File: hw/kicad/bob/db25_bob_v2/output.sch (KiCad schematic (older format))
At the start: 6 parts, among them P5 CONN_01X08, P6 CONN_01X08, P7 CONN_01X08, P8 CONN_01X08, U18 NCV7608, U19 NCV7608

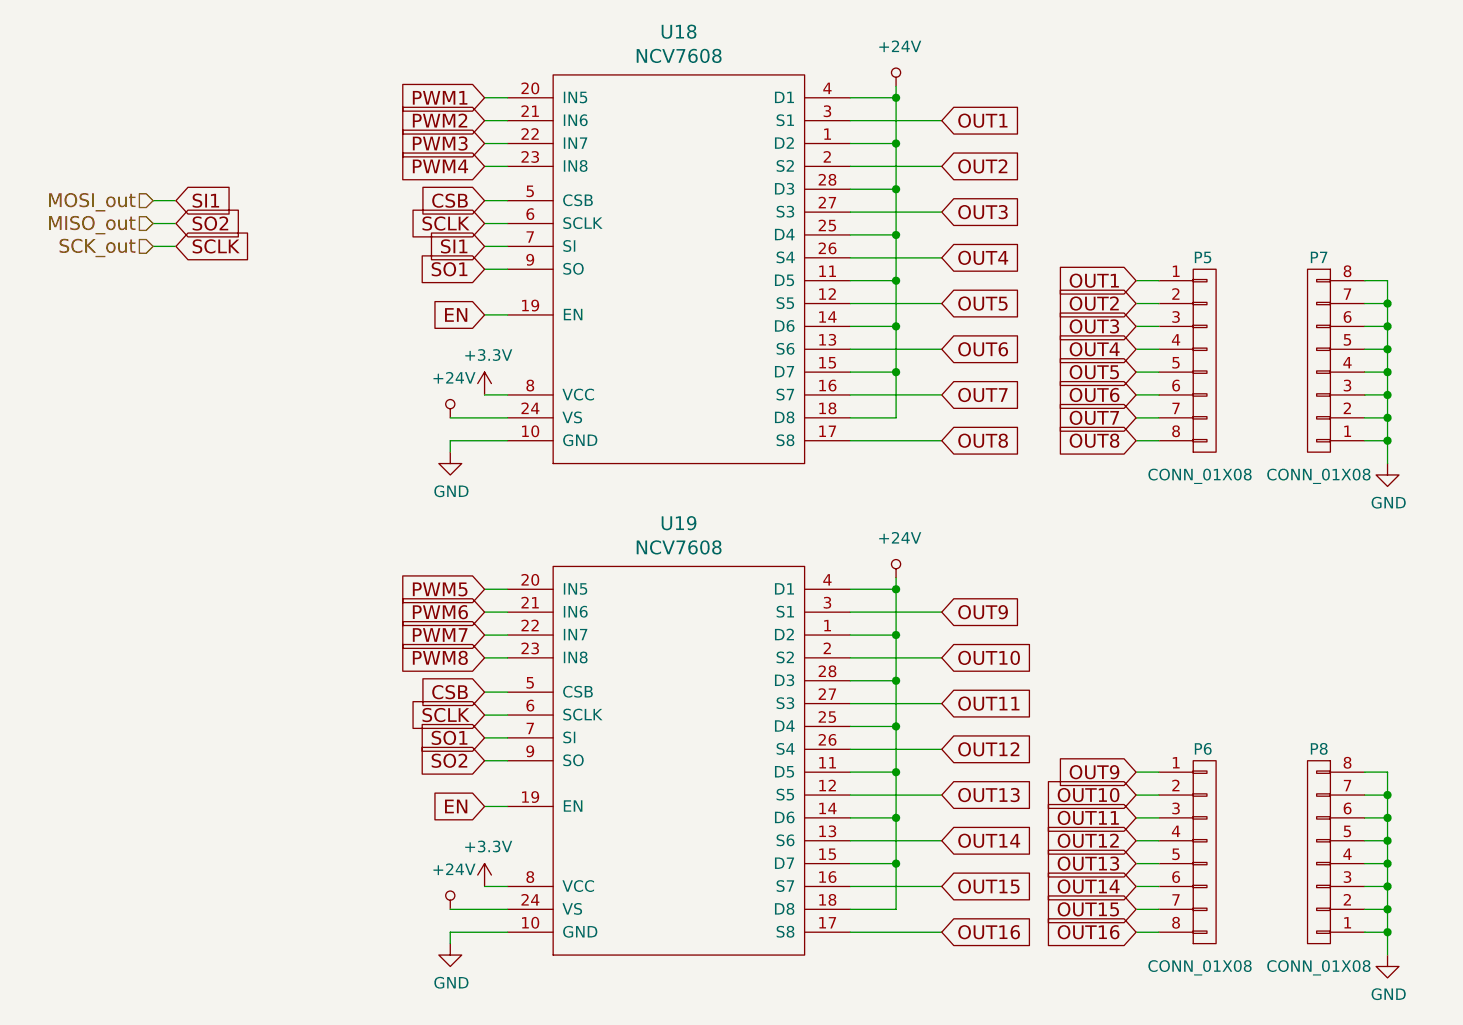
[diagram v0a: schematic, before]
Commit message: More stuff.
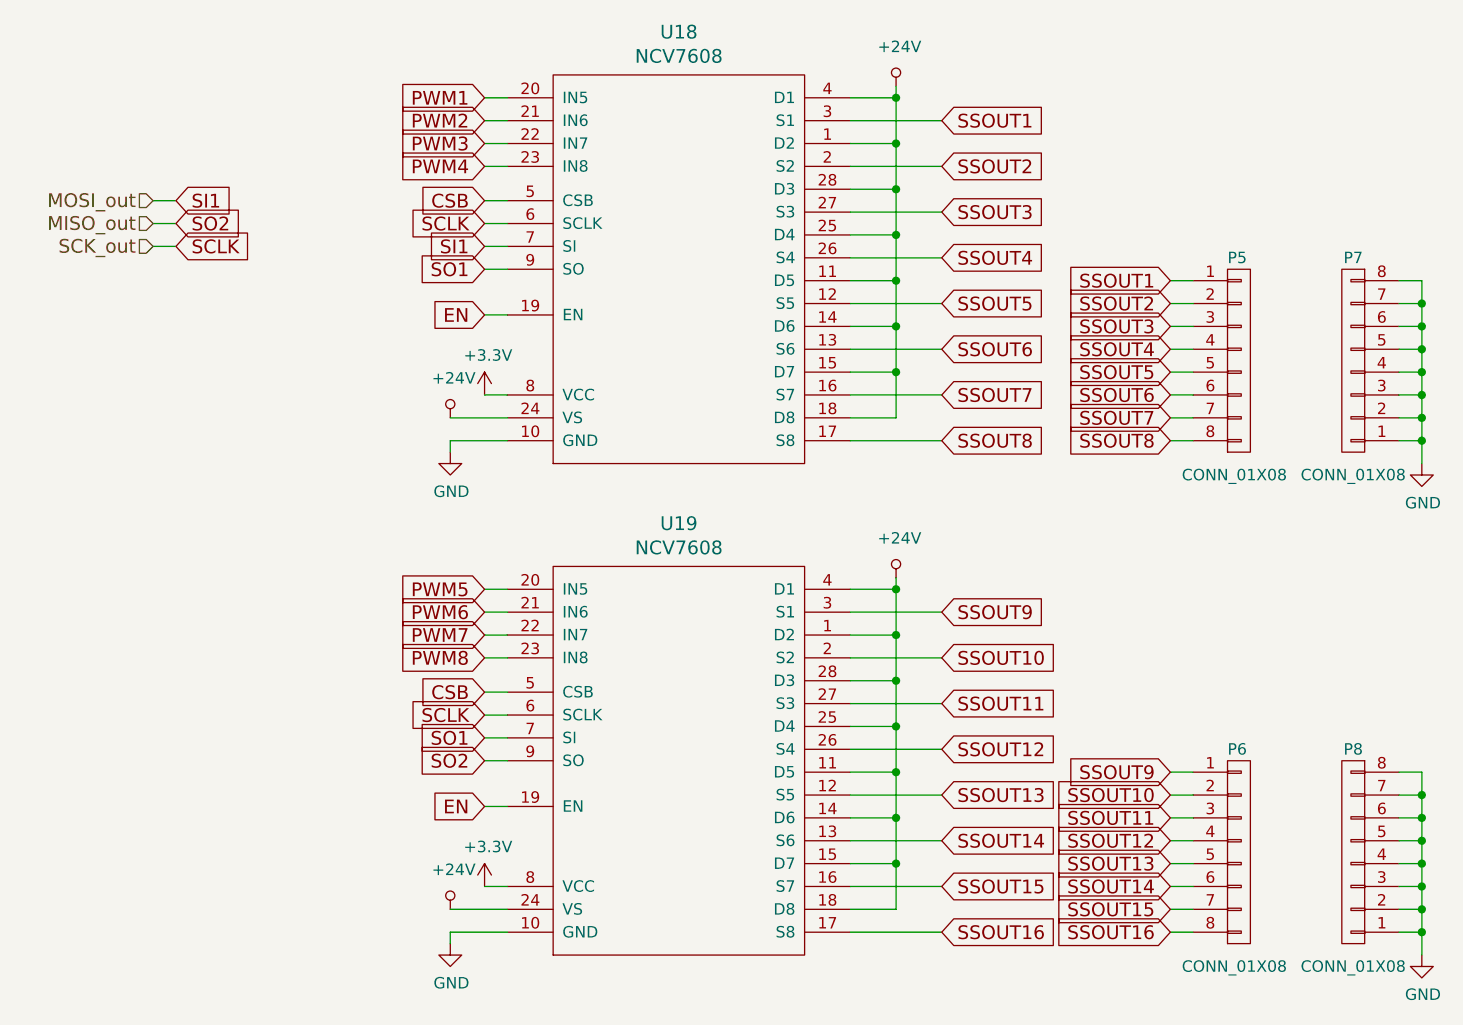
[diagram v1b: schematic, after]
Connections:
- net OUT1 renamed SSOUT1
- net OUT10 renamed SSOUT10
- net OUT11 renamed SSOUT11
- net OUT12 renamed SSOUT12
- net OUT13 renamed SSOUT13
- net OUT14 renamed SSOUT14
- net OUT15 renamed SSOUT15
- net OUT16 renamed SSOUT16
- net OUT2 renamed SSOUT2
- net OUT3 renamed SSOUT3
- net OUT4 renamed SSOUT4
- net OUT5 renamed SSOUT5
- net OUT6 renamed SSOUT6
- net OUT7 renamed SSOUT7
- net OUT8 renamed SSOUT8
- net OUT9 renamed SSOUT9
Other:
- moved on the sheet: P5, P6, P7, P8

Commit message: Wip
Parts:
- P5, P6, P7, P8: footprint Terminal_Blocks:TerminalBlock_Pheonix_PT-3.5mm_8pol -> Terminal_Blocks:TerminalBlock_Pheonix_MPT-2.54mm_8pol
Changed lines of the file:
@@
 $EndComp
 $Comp
-L +24V #PWR068
+L +24V #PWR039
 U 1 1 57449F65
 P 3100 3150
-F 0 "#PWR068" H 3100 3000 50  0001 C CNN
+F 0 "#PWR039" H 3100 3000 50  0001 C CNN
 F 1 "+24V" H 3115 3323 50  0000 C CNN
 F 2 "" H 3100 3150 50  0000 C CNN
@@
 P 3100 3300
 AR Path="/57449FA2" Ref="#PWR027"  Part="1"
-AR Path="/5744969F/57449FA2" Ref="#PWR069"  Part="1"
-F 0 "#PWR069" H 3100 3050 50  0001 C CNN
+AR Path="/5744969F/57449FA2" Ref="#PWR040"  Part="1"
+F 0 "#PWR040" H 3100 3050 50  0001 C CNN
 F 1 "GND" H 3105 3127 50  0000 C CNN
 F 2 "" H 3100 3300 50  0000 C CNN
@@
 P 3250 3050
 AR Path="/57449FDD" Ref="#PWR028"  Part="1"
-AR Path="/5744969F/57449FDD" Ref="#PWR070"  Part="1"
-F 0 "#PWR070" H 3250 2900 50  0001 C CNN
+AR Path="/5744969F/57449FDD" Ref="#PWR041"  Part="1"
+F 0 "#PWR041" H 3250 2900 50  0001 C CNN
 F 1 "+3.3V" H 3265 3223 50  0000 C CNN
 F 2 "" H 3250 3050 50  0000 C CNN
@@
 PWM4
 $Comp
-L +24V #PWR071
+L +24V #PWR042
 U 1 1 5744A372
 P 5050 1700
-F 0 "#PWR071" H 5050 1550 50  0001 C CNN
+F 0 "#PWR042" H 5050 1550 50  0001 C CNN
 F 1 "+24V" H 5065 1873 50  0000 C CNN
 F 2 "" H 5050 1700 50  0000 C CNN
@@
 F 0 "P5" H 6500 3350 50  0000 L CNN
 F 1 "CONN_01X08" H 6300 2400 50  0000 L CNN
-F 2 "Terminal_Blocks:TerminalBlock_Pheonix_PT-3.5mm_8pol" H 6550 2900 50  0001 C CNN
+F 2 "Terminal_Blocks:TerminalBlock_Pheonix_MPT-2.54mm_8pol" H 6550 2900 50  0001 C CNN
 F 3 "" H 6550 2900 50  0000 C CNN
 	1    6550 2900
@@
 F 0 "P7" H 7050 2450 50  0000 C CNN
 F 1 "CONN_01X08" H 7050 3400 50  0000 C CNN
-F 2 "Terminal_Blocks:TerminalBlock_Pheonix_PT-3.5mm_8pol" H 7050 2900 50  0001 C CNN
+F 2 "Terminal_Blocks:TerminalBlock_Pheonix_MPT-2.54mm_8pol" H 7050 2900 50  0001 C CNN
 F 3 "" H 7050 2900 50  0000 C CNN
 	1    7050 2900
@@
 P 7350 3350
 AR Path="/5744AAA7" Ref="#PWR030"  Part="1"
-AR Path="/5744969F/5744AAA7" Ref="#PWR072"  Part="1"
-F 0 "#PWR072" H 7350 3100 50  0001 C CNN
+AR Path="/5744969F/5744AAA7" Ref="#PWR043"  Part="1"
+F 0 "#PWR043" H 7350 3100 50  0001 C CNN
 F 1 "GND" H 7355 3177 50  0000 C CNN
 F 2 "" H 7350 3350 50  0000 C CNN
@@
 $EndComp
 $Comp
-L +24V #PWR073
+L +24V #PWR044
 U 1 1 5744AECC
 P 3100 5300
-F 0 "#PWR073" H 3100 5150 50  0001 C CNN
+F 0 "#PWR044" H 3100 5150 50  0001 C CNN
 F 1 "+24V" H 3115 5473 50  0000 C CNN
 F 2 "" H 3100 5300 50  0000 C CNN
@@
 P 3100 5450
 AR Path="/5744AED2" Ref="#PWR032"  Part="1"
-AR Path="/5744969F/5744AED2" Ref="#PWR074"  Part="1"
-F 0 "#PWR074" H 3100 5200 50  0001 C CNN
+AR Path="/5744969F/5744AED2" Ref="#PWR045"  Part="1"
+F 0 "#PWR045" H 3100 5200 50  0001 C CNN
 F 1 "GND" H 3105 5277 50  0000 C CNN
 F 2 "" H 3100 5450 50  0000 C CNN
@@
 P 3250 5200
 AR Path="/5744AED8" Ref="#PWR033"  Part="1"
-AR Path="/5744969F/5744AED8" Ref="#PWR075"  Part="1"
-F 0 "#PWR075" H 3250 5050 50  0001 C CNN
+AR Path="/5744969F/5744AED8" Ref="#PWR046"  Part="1"
+F 0 "#PWR046" H 3250 5050 50  0001 C CNN
 F 1 "+3.3V" H 3265 5373 50  0000 C CNN
 F 2 "" H 3250 5200 50  0000 C CNN
@@
 PWM5
 $Comp
-L +24V #PWR076
+L +24V #PWR047
 U 1 1 5744AEE7
 P 5050 3850
-F 0 "#PWR076" H 5050 3700 50  0001 C CNN
+F 0 "#PWR047" H 5050 3700 50  0001 C CNN
 F 1 "+24V" H 5065 4023 50  0000 C CNN
 F 2 "" H 5050 3850 50  0000 C CNN
@@
 F 0 "P6" H 6500 5500 50  0000 L CNN
 F 1 "CONN_01X08" H 6300 4550 50  0000 L CNN
-F 2 "Terminal_Blocks:TerminalBlock_Pheonix_PT-3.5mm_8pol" H 6550 5050 50  0001 C CNN
+F 2 "Terminal_Blocks:TerminalBlock_Pheonix_MPT-2.54mm_8pol" H 6550 5050 50  0001 C CNN
 F 3 "" H 6550 5050 50  0000 C CNN
 	1    6550 5050
@@
 F 0 "P8" H 7050 4600 50  0000 C CNN
 F 1 "CONN_01X08" H 7050 5550 50  0000 C CNN
-F 2 "Terminal_Blocks:TerminalBlock_Pheonix_PT-3.5mm_8pol" H 7050 5050 50  0001 C CNN
+F 2 "Terminal_Blocks:TerminalBlock_Pheonix_MPT-2.54mm_8pol" H 7050 5050 50  0001 C CNN
 F 3 "" H 7050 5050 50  0000 C CNN
 	1    7050 5050
@@
 P 7350 5500
 AR Path="/5744AF3F" Ref="#PWR035"  Part="1"
-AR Path="/5744969F/5744AF3F" Ref="#PWR077"  Part="1"
-F 0 "#PWR077" H 7350 5250 50  0001 C CNN
+AR Path="/5744969F/5744AF3F" Ref="#PWR048"  Part="1"
+F 0 "#PWR048" H 7350 5250 50  0001 C CNN
 F 1 "GND" H 7355 5327 50  0000 C CNN
 F 2 "" H 7350 5500 50  0000 C CNN
